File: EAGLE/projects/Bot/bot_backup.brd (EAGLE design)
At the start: 160 x 100 mm, 18 parts, among them IC1 7805T, U3 ARDUINO_SHIELDLABEL

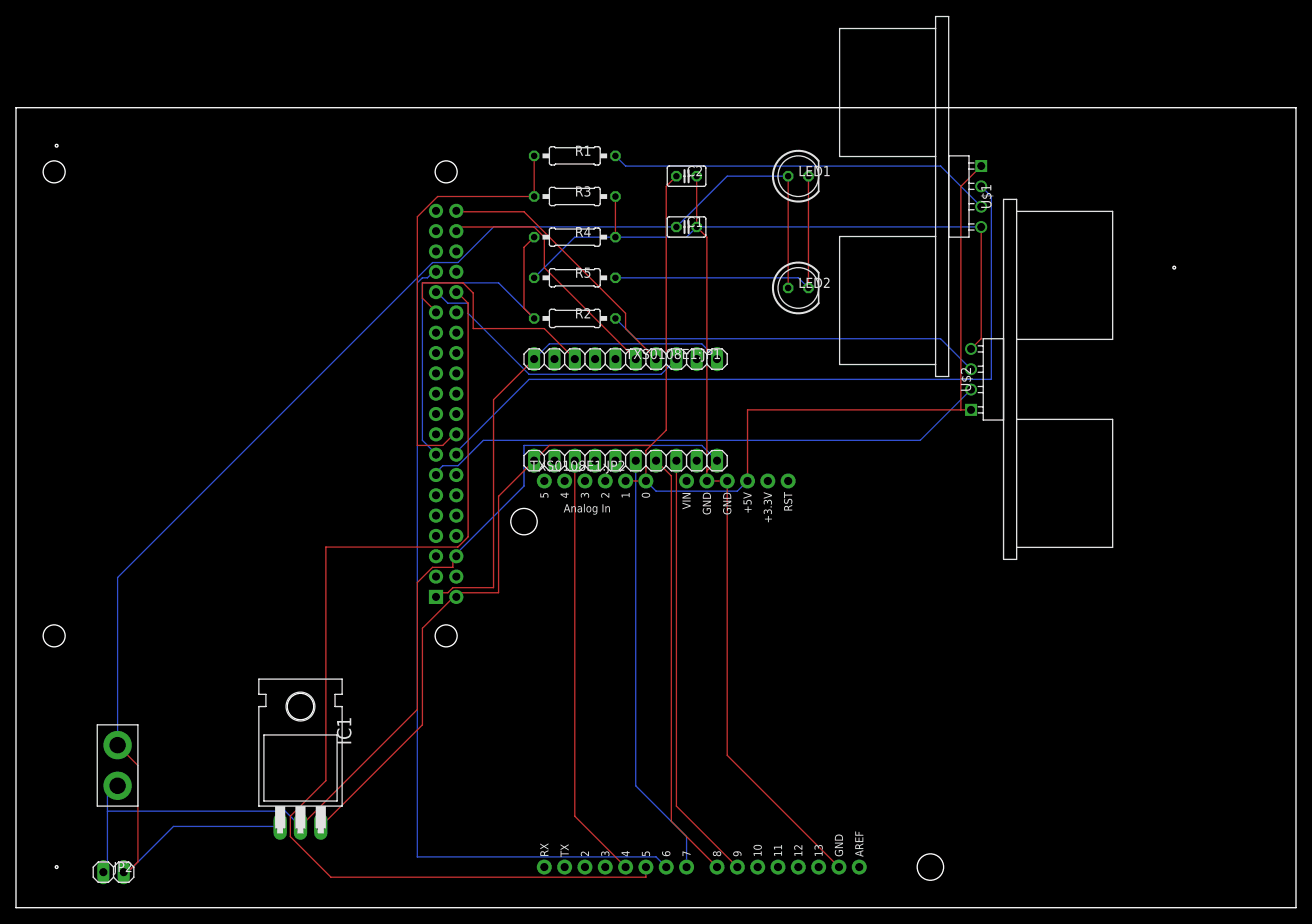
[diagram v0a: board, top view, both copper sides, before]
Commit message: Ready to mill
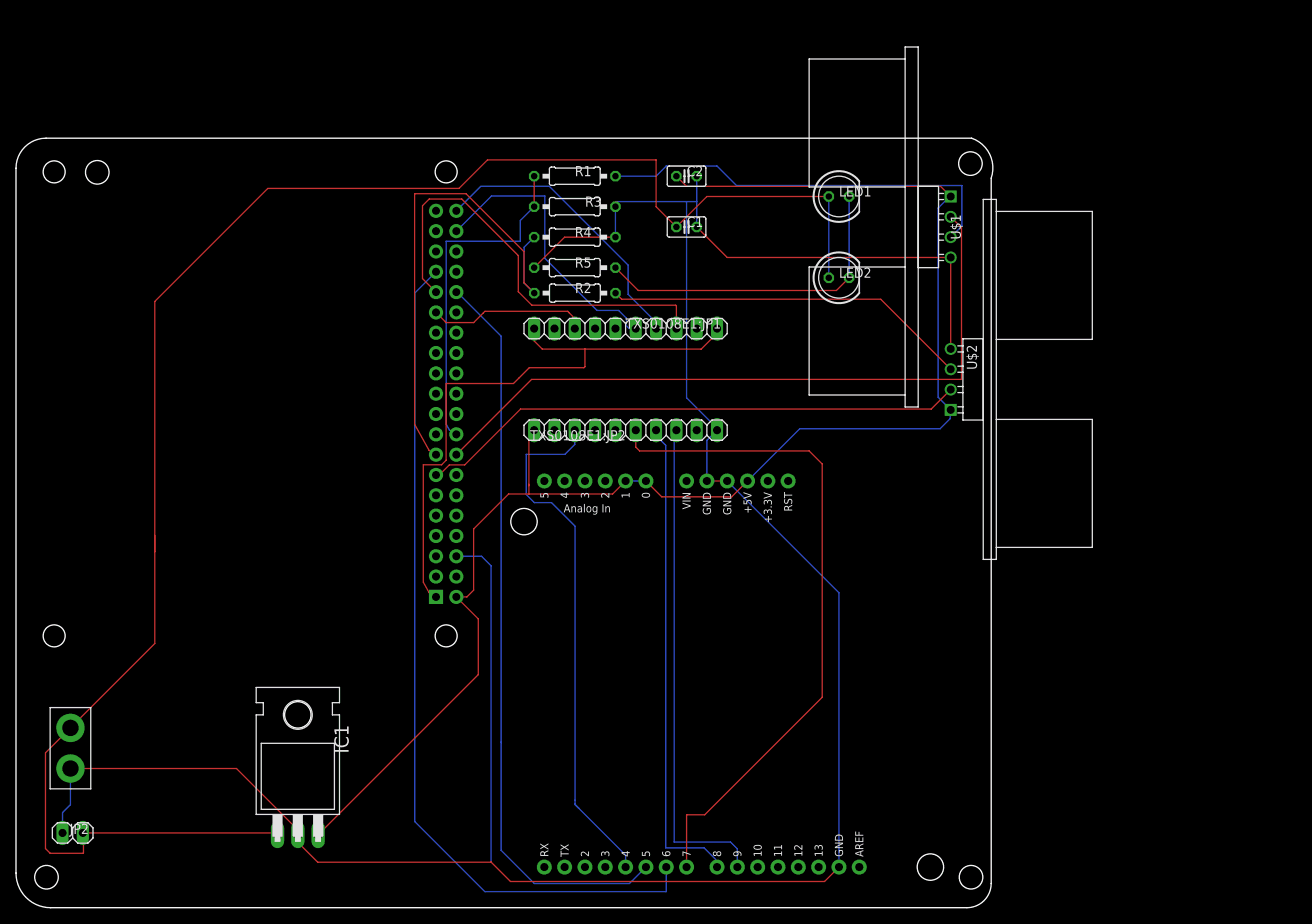
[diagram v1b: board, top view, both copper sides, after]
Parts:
- R5: value 1k -> 10
- moved JP2 7.08 mm to (7.09, 9.35)
- moved JP7 6.28 mm to (6.81, 19.9)
- moved LED1 5.68 mm to (102.9, 88.9)
- moved U$1 5.39 mm to (116.8, 85.1)
- moved LED2 5.24 mm to (102.9, 78.7)
- moved TXS0108E1:JP1 3.81 mm to (76.2, 72.4)
- moved TXS0108E1:JP2 3.81 mm to (76.2, 59.7)
- moved R2 3.17 mm to (69.9, 76.8)
- moved R1 2.54 mm to (69.8, 91.4)
- moved U$2 2.54 mm to (116.8, 66.0)
- moved R3 1.27 mm to (69.8, 87.6)
- moved R5 1.27 mm to (69.8, 80.0)
- moved IC1 1.09 mm to (35.2, 19.3)
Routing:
- net L_SPD: track 135.4 -> 92.9 mm
- net PWR+: track 179.4 -> 218.3 mm
- net N$14: track 53.4 -> 85.1 mm
- net 0: track 299.6 -> 325.0 mm
- net R_BCK: track 35.8 -> 54.6 mm
- net R_US_ECHO: track 49.2 -> 64.0 mm
- net N$13: track 53.4 -> 67.1 mm
- net PI_3V3: track 62.9 -> 76.5 mm
- net L_US_ECHO: track 54.7 -> 42.8 mm
- net PI_5V: track 199.6 -> 189.1 mm
- net R_FWD: track 30.0 -> 20.1 mm
- net N$16: track 54.0 -> 62.1 mm
- net L_US_TRIG: track 95.6 -> 87.9 mm
- net N$15: track 54.0 -> 60.6 mm
- net L_FWD: track 31.9 -> 36.4 mm
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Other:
- board size 160 x 100 mm -> 122.1 x 96.2 mm
